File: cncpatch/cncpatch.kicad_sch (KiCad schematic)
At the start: 40 parts, among them J1 Conn_01x03_Socket, J2 Conn_01x03_Socket, J3 Conn_01x03_Socket, J4 Conn_01x03_Socket, J5 Conn_01x03_Socket, J6 Conn_01x03_Socket, J7 Conn_01x08_Socket, Q1 BC858, Q2 BC858, Q3 BC858, Q4 AO3401A, U2 PC817

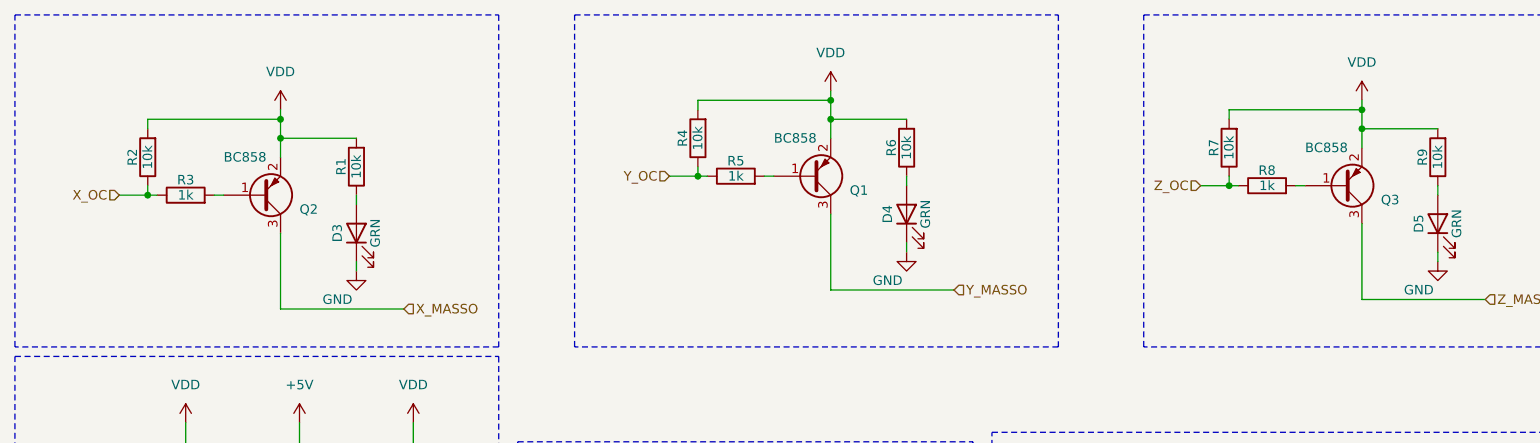
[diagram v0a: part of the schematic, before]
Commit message: Typos and reord
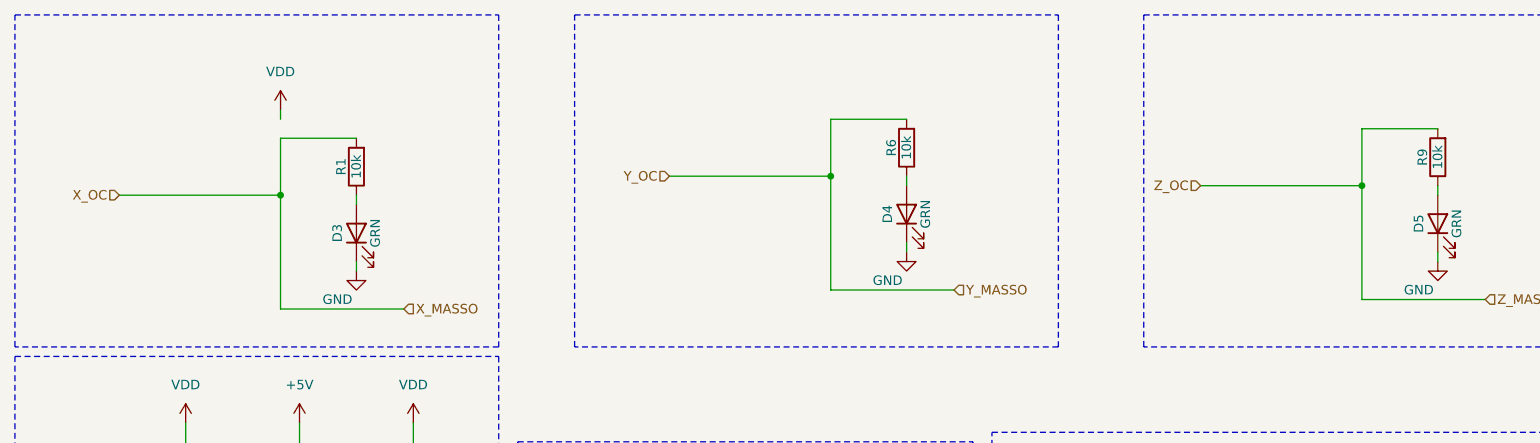
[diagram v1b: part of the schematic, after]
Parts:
- removed Q1, Q2, Q3: BC858, Package_TO_SOT_SMD:SOT-23, symbol Transistor_BJT:BC858
- removed R2, R4, R7: 10k, Resistor_SMD:R_0603_1608Metric, symbol Device:R
- removed R3, R5, R8: 1k, Resistor_SMD:R_0603_1608Metric, symbol Device:R
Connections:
- net X_OC is gone; now on net X_MASSO: J1.2 (Pin_2)
- net Y_OC is gone; now on net Y_MASSO: J3.2 (Pin_2)
- net Z_OC is gone; now on net Z_MASSO: J5.2 (Pin_2)
- net VDD: no longer R1.2, R6.2, R9.2
- net X_MASSO: now also R1.2
- net Y_MASSO: now also R6.2
- net Z_MASSO: now also R9.2
